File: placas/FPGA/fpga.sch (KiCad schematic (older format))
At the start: 46 parts, among them IC1 XCF01S-VO20, K1 MODE_PROG, P1 A, P2 B, P3 JTAG, P4 POWER, P5 PUDC, SW1 RESET_PROG, U1 XC3S50A-VQ100, U2 TPS75003_PM

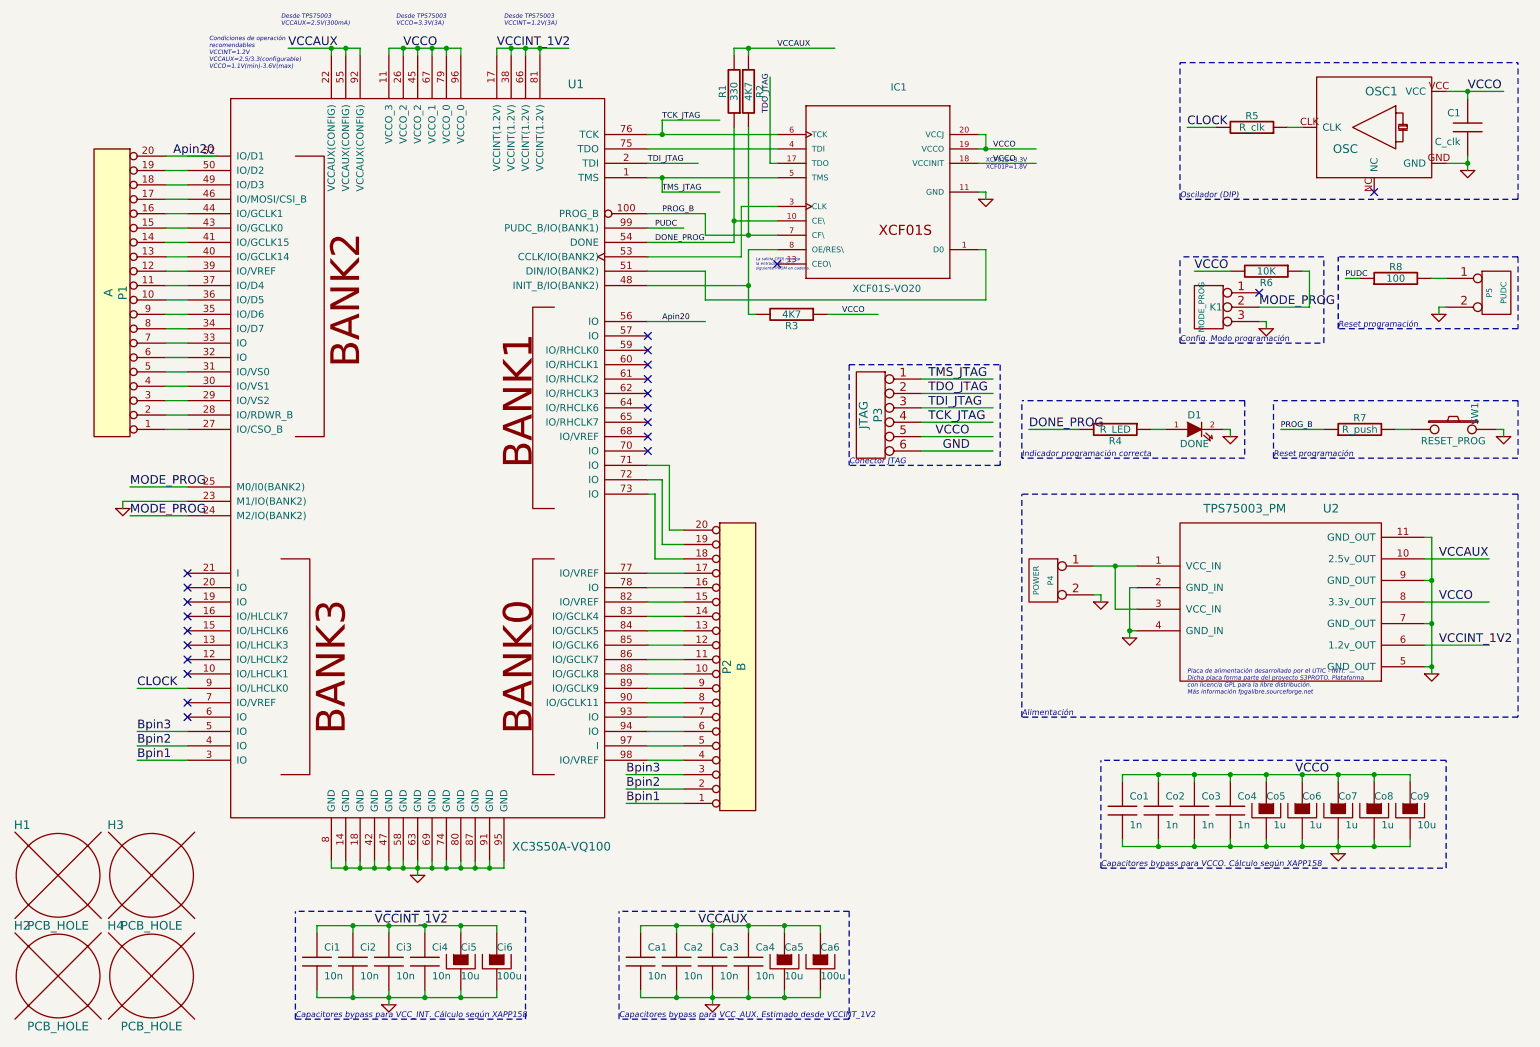
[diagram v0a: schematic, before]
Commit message: [PLACA]se corrige los errores en la signacion de pines, además se agrega el pin 52 en el esquemático
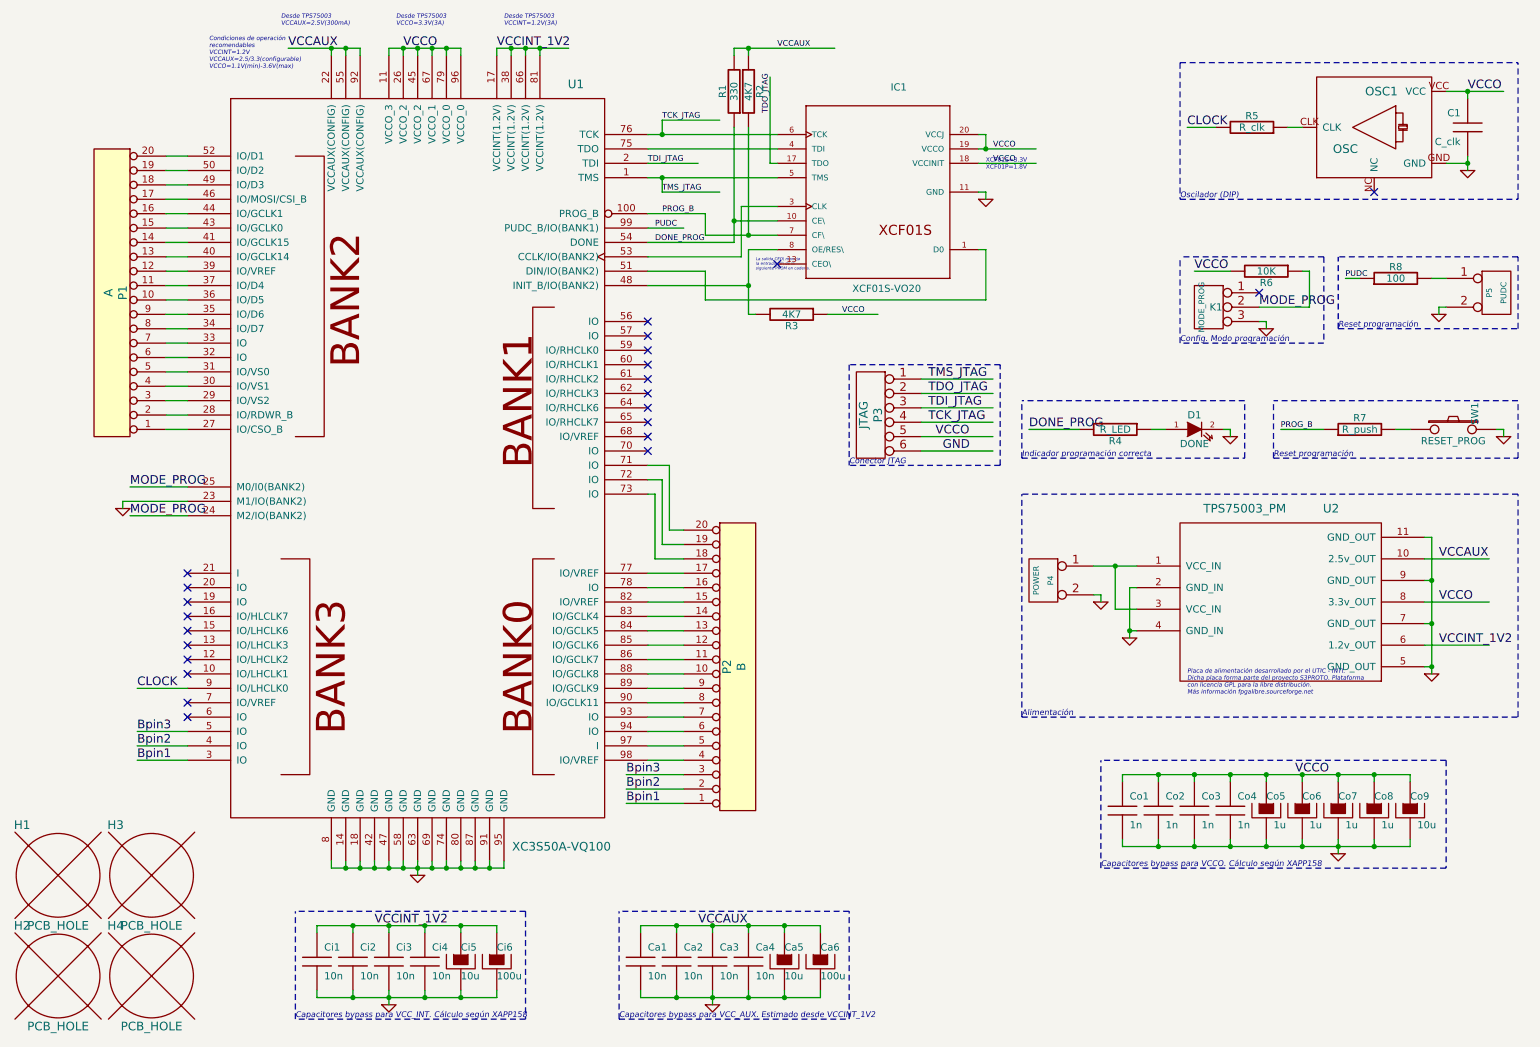
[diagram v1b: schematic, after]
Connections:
- net labels removed: Apin20
- wire segments 219 -> 218
- no-connect marks 22 -> 23
